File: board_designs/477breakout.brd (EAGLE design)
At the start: 104.2 x 49.5 mm, 22 parts, among them IC1 PIC24FJ128GA006, J1 RJ11-6PTH, J2 5.5x2.1mm Barrel, U2 3.3V/150mA, U3 5V

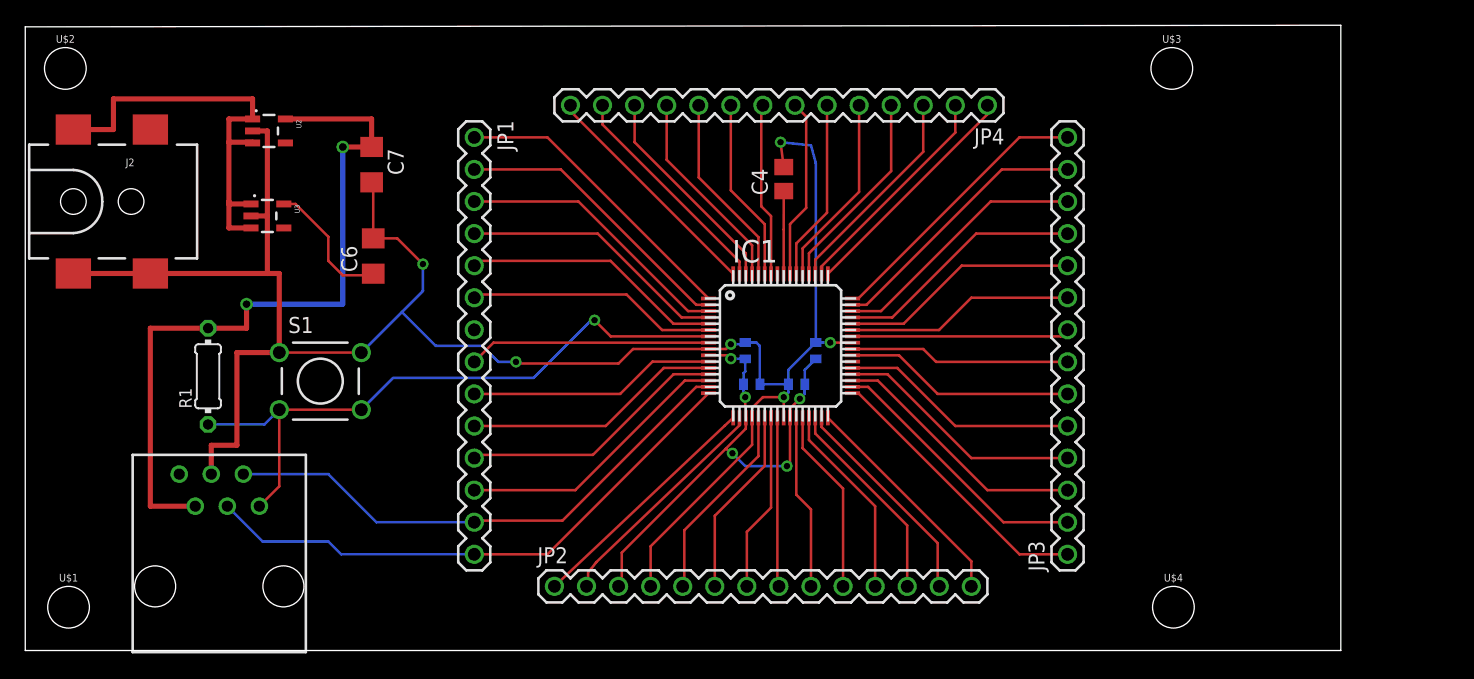
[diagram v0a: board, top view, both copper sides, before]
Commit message: Updated board designs
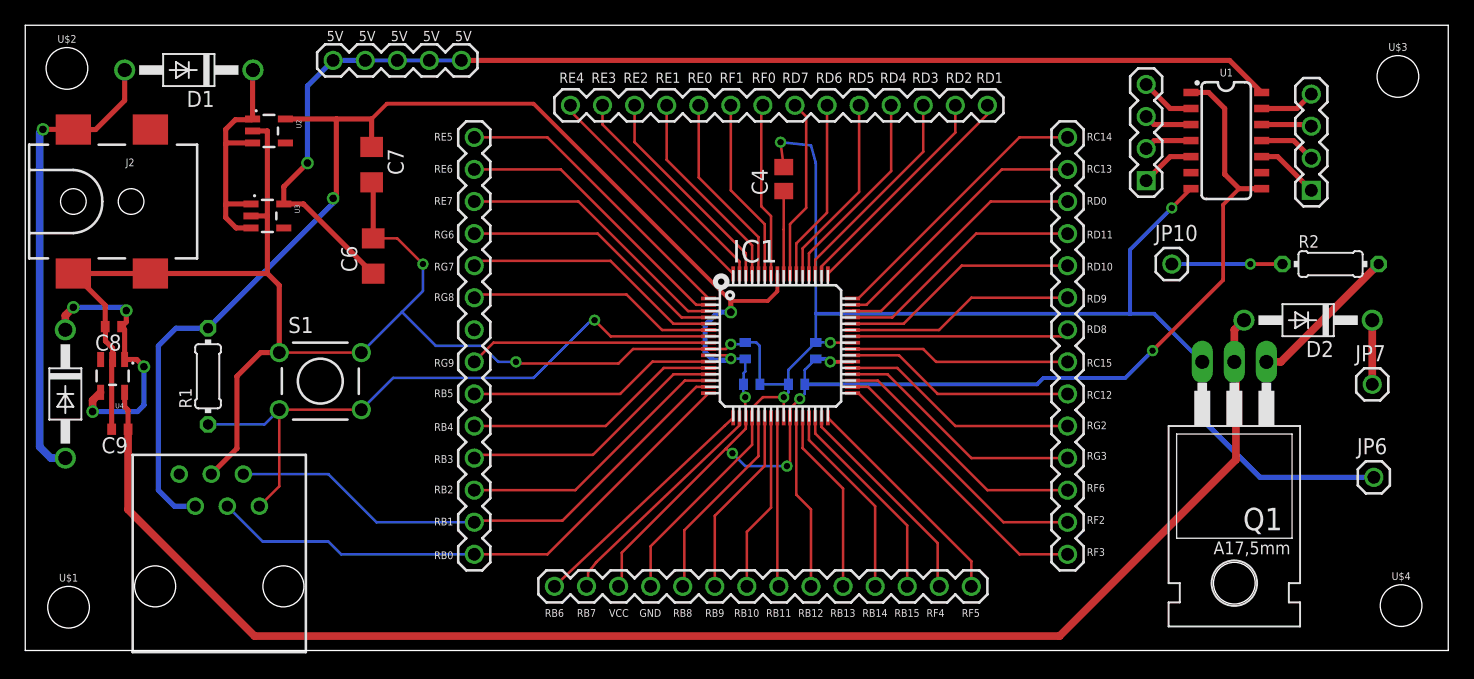
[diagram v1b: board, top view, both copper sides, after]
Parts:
- added C8, C9: 1 uF, rcl:C0402
- added D1, D2, D3: 1N4004, diode:DO41-10
- added JP10: M01PTH, SparkFun:1X01
- added JP5: (no value), SparkFun:1X05
- added JP6: GND, SparkFun:1X01
- added JP7: 12V, SparkFun:1X01
- added JP8, JP9: (no value), SparkFun:1X04
- added Q1: TIP120, transistor-power:TO220AH
- added R2: 1K, rcl:0204/7
- added U1: TXB0104, SparkFun-IC-Comms:SO14
- added U4: V_REG_MIC5205RT9069, SparkFun-IC-Power:SOT23-5
- C6, C7: value (none) -> 2.2 uF
- moved U$4 18.0 mm to (109.0, 3.56)
- moved U$3 17.9 mm to (108.7, 45.5)
- moved U$2 0.13 mm to (3.30, 46.1)
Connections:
- new net 12V: C9.1, D2.A, Q1.C, U4.5
- new net N$10: JP9.1, U1.10
- new net N$11: D1.A, D3.A, J2.VIN0
- new net N$12: Q1.B, R2.2
- new net N$14: D2.C, JP7.1
- new net N$15: JP10.1, R2.1
- new net N$16: C8.1, D3.C, U4.1, U4.4
- new net N$3: JP8.4, U1.2
- new net N$4: JP8.3, U1.3
- new net N$5: JP8.2, U1.4
- new net N$6: JP8.1, U1.5
- new net N$7: JP9.4, U1.13
- new net N$8: JP9.3, U1.12
- new net N$9: JP9.2, U1.11
- net 5V: now also JP5.1, JP5.2, JP5.3, JP5.4, JP5.5, U1.14
- net GND: now also C8.2, C9.2, JP6.1, Q1.E, U1.7, U4.2
- net N$2: now also D1.C; no longer J2.VIN0
- net VCC: now also U1.1, U1.8
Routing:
- net 12V: track 0.00 -> 118.5 mm
- net VCC: track 98.9 -> 197.5 mm, vias 7 -> 9
- net 5V: track 10.6 -> 96.9 mm, vias 0 -> 1
- net GND: track 162.6 -> 237.6 mm, vias 6 -> 7
- net N$11: track 0.00 -> 37.5 mm, vias 0 -> 1
- net N$16: track 0.00 -> 21.3 mm, vias 0 -> 4
- net N$2: track 34.3 -> 19.9 mm
- net N$12: track 0.00 -> 12.1 mm
- net N$15: track 0.00 -> 8.76 mm, vias 0 -> 1
- net N$14: track 0.00 -> 5.08 mm
- net N$10: track 0.00 -> 5.04 mm
- net N$9: track 0.00 -> 4.51 mm
- net N$7: track 0.00 -> 4.40 mm
- net N$6: track 0.00 -> 4.34 mm
- net N$3: track 0.00 -> 4.34 mm
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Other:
- board size 104.2 x 49.5 mm -> 112.7 x 49.5 mm
- board text added: "5V"
- board text added: "GND"
- board text added: "RB0"
- board text added: "RB1"
- board text added: "RB10"
- board text added: "RB11"
- board text added: "RB12"
- board text added: "RB13"
- board text added: "RB14"
- board text added: "RB15"
- board text added: "RB2"
- board text added: "RB3"
- board text added: "RB4"
- board text added: "RB5"
- board text added: "RB6"
- board text added: "RB7"
- board text added: "RB8"
- board text added: "RB9"
- board text added: "RC12"
- board text added: "RC13"
- board text added: "RC14"
- board text added: "RC15"
- board text added: "RD0"
- board text added: "RD1"
- board text added: "RD10"
- board text added: "RD11"
- board text added: "RD2"
- board text added: "RD3"
- board text added: "RD4"
- board text added: "RD5"
- board text added: "RD6"
- board text added: "RD7"
- board text added: "RD8"
- board text added: "RD9"
- board text added: "RE0"
- board text added: "RE1"
- board text added: "RE2"
- board text added: "RE3"
- board text added: "RE4"
- board text added: "RE5"
- board text added: "RE6"
- board text added: "RE7"
- board text added: "RF0"
- board text added: "RF1"
- board text added: "RF2"
- board text added: "RF3"
- board text added: "RF4"
- board text added: "RF5"
- board text added: "RF6"
- board text added: "RG2"
- board text added: "RG3"
- board text added: "RG6"
- board text added: "RG7"
- board text added: "RG8"
- board text added: "RG9"
- board text added: "VCC"
